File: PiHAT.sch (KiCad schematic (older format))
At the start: 17 parts, among them U1 LM2596T-ADJ

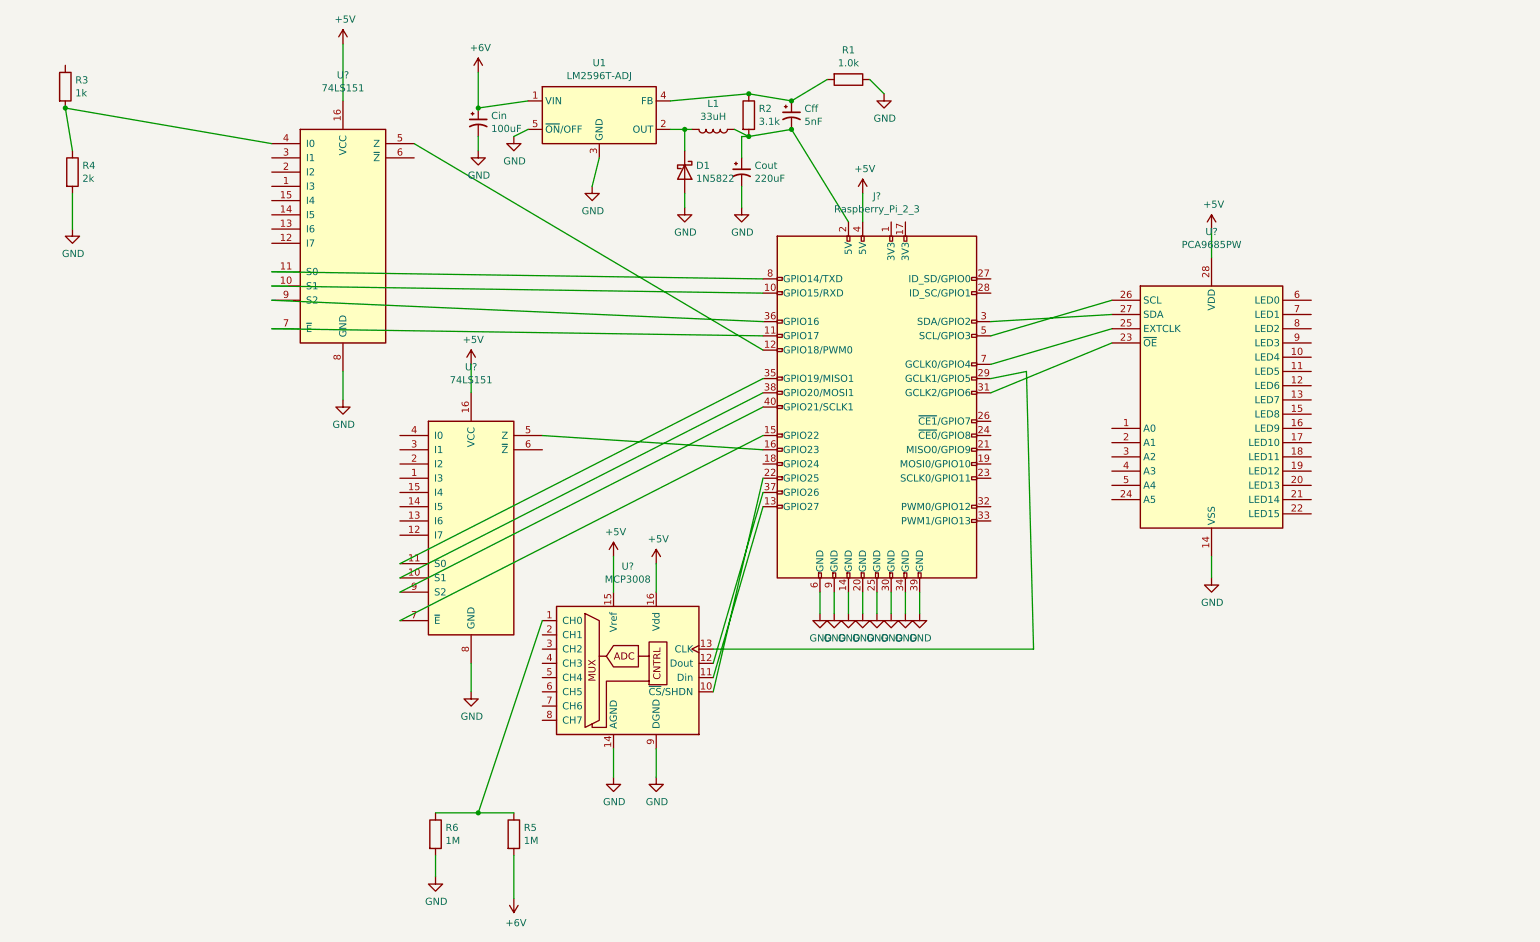
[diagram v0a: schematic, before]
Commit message: Add files via upload
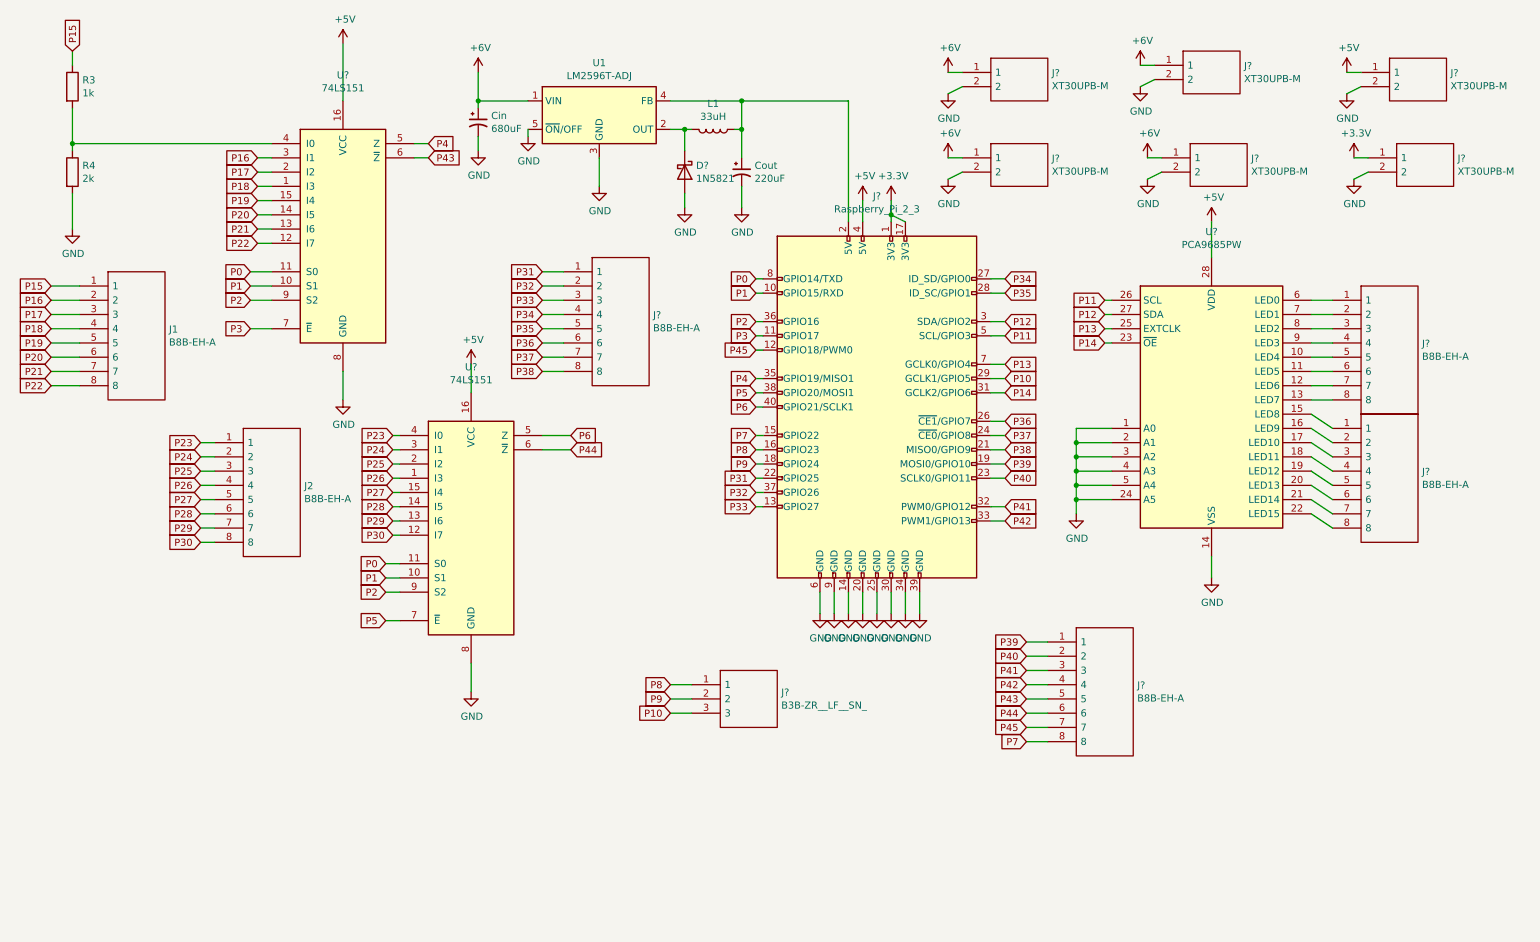
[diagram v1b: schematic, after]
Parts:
- removed Cff: 5nF, symbol Device:CP1_Small
- removed D1: 1N5822, Diode_THT:D_DO-201AD_P15.24mm_Horizontal, symbol Diode:1N5822
- removed R1: 1.0k, symbol Device:R
- removed R2: 3.1k, symbol Device:R
- removed R5, R6: 1M, symbol Device:R
- removed U?: MCP3008, symbol Analog_ADC:MCP3008
- added D?: 1N5821, Diode_THT:D_DO-201AD_P15.24mm_Horizontal, symbol Diode:1N5821
- added J1, J2, J? (x4): B8B-EH-A, SHDR8W64P0X250_1X8_2250X380X600P, symbol SamacSys_Parts:B8B-EH-A
- added J? (x6): XT30UPB-M, SHDR2W160P0X500_1X2_1020X520X1070P, symbol XT30UPB-M:XT30UPB-M
- added J?: B3B-ZR__LF__SN_, SHDR3W50P0X150_1X3_600X350X450P, symbol B3B-ZR__LF__SN_:B3B-ZR__LF__SN_
- Cin: value 100uF -> 680uF
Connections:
- net +5V: now also J?.1
- net +6V: now also J?.1, J?.1, J?.1, J?.1
- net GND: now also U?.1 (A0), U?.2 (A1), U?.24 (A5), U?.3 (A2), U?.4 (A3), U?.5 (A4), D?.2 (A), J?.2, J?.2, J?.2, J?.2, J?.2, J?.2
- net P26: now reaches U?.1 (I3)
- net P26: now also J2.4
- net P1: now reaches U?.10 (S1)
- net P1: now also J?.10 (GPIO15/RXD), U?.10 (S1); no longer J?.38 (GPIO20/MOSI1)
- net P0: now reaches U?.11 (S0)
- net P0: now also J?.8 (GPIO14/TXD), U?.11 (S0); no longer J?.35 (GPIO19/MISO1)
- net P30: now reaches U?.12 (I7)
- net P30: now also J2.8
- net P29: now reaches U?.13 (I6)
- net P29: now also J2.7
- net P28: now reaches U?.14 (I5)
- net P28: now also J2.6
- net P27: now reaches U?.15 (I4)
- net P27: now also J2.5
- net P25: now reaches U?.2 (I2)
- net P25: now also J2.3
- net P24: now reaches U?.3 (I1)
- net P24: now also J2.2
- net P23: now reaches U?.4 (I0)
- net P23: now also J2.1
- net P6: now reaches U?.5 (Z)
- net P6: now also J?.40 (GPIO21/SCLK1); no longer J?.16 (GPIO23)
- net P44: now reaches U?.6 (~Z)
- net P44: now also J?.6
- net P5: now reaches U?.7 (~E)
- net P5: now also J?.38 (GPIO20/MOSI1); no longer J?.15 (GPIO22)
- net P2: now reaches U?.9 (S2)
- net P2: now also J?.36 (GPIO16), U?.9 (S2); no longer J?.40 (GPIO21/SCLK1)
- net P18: now reaches U?.1 (I3)
- net P18: now also J1.4
- net P22: now reaches U?.12 (I7)
- net P22: now also J1.8
- net P21: now reaches U?.13 (I6)
- net P21: now also J1.7
- net P20: now reaches U?.14 (I5)
- net P20: now also J1.6
- net P19: now reaches U?.15 (I4)
- net P19: now also J1.5
- net P17: now reaches U?.2 (I2)
- net P17: now also J1.3
- net P16: now reaches U?.3 (I1)
- net P16: now also J1.2
- net P4: now reaches U?.5 (Z)
- net P4: now also J?.35 (GPIO19/MISO1); no longer J?.12 (GPIO18/PWM0)
- net P43: now reaches U?.6 (~Z)
- net P43: now also J?.5
- net P3: now reaches J?.11 (GPIO17), U?.7 (~E)
- net +3V3: now reaches J?.1 (3V3)
- net +3V3: now also J?.17 (3V3), J?.1
- net P33: now reaches J?.13 (GPIO27)
- net P33: now also J?.3
- net P9: now reaches J?.18 (GPIO24)
- net P9: now also J?.2
- net P39: now reaches J?.19 (MOSI0/GPIO10)
- net P39: now also J?.1
- net at Cout.1, J?.2 (5V), L1.1: now also U1.4 (FB)
- net P38: now reaches J?.21 (MISO0/GPIO9)
- net P38: now also J?.8
- net P31: now reaches J?.22 (GPIO25)
- net P31: now also J?.1
- net P40: now reaches J?.23 (SCLK0/GPIO11)
- net P40: now also J?.2
- net P37: now reaches J?.24 (~CE0~/GPIO8)
- net P37: now also J?.7
- net P36: now reaches J?.26 (~CE1~/GPIO7)
- net P36: now also J?.6
- net P34: now reaches J?.27 (ID_SD/GPIO0)
- net P34: now also J?.4
- net P35: now reaches J?.28 (ID_SC/GPIO1)
- net P35: now also J?.5
- net P10: now reaches J?.29 (GCLK1/GPIO5)
- net P10: now also J?.3
- net P12: now reaches J?.3 (SDA/GPIO2), U?.27 (SDA)
- net P14: now reaches J?.31 (GCLK2/GPIO6), U?.23 (~OE)
- net P41: now reaches J?.32 (PWM0/GPIO12)
- net P41: now also J?.3
- net P42: now reaches J?.33 (PWM1/GPIO13)
- net P42: now also J?.4
- net P32: now reaches J?.37 (GPIO26)
- net P32: now also J?.2
- net P11: now reaches J?.5 (SCL/GPIO3), U?.26 (SCL)
- net P13: now reaches J?.7 (GCLK0/GPIO4), U?.25 (EXTCLK)
- net at L1.2, U1.2 (OUT): now also D?.1 (K)
- net P15: now reaches R3.1
- net P15: now also J1.1
- net at U?.10 (LED4): now also J?.5
- net at U?.11 (LED5): now also J?.6
- net at U?.12 (LED6): now also J?.7
- net at U?.13 (LED7): now also J?.8
- net at U?.15 (LED8): now also J?.1
- net at U?.16 (LED9): now also J?.2
- net at U?.17 (LED10): now also J?.3
- net at U?.18 (LED11): now also J?.4
- net at U?.19 (LED12): now also J?.5
- net at U?.20 (LED13): now also J?.6
- net at U?.21 (LED14): now also J?.7
- net at U?.22 (LED15): now also J?.8
- net at U?.6 (LED0): now also J?.1
- net at U?.7 (LED1): now also J?.2
- net at U?.8 (LED2): now also J?.3
- net at U?.9 (LED3): now also J?.4
- new net P45: J?.12 (GPIO18/PWM0), J?.7
- new net P7: J?.15 (GPIO22), J?.8
- new net P8: J?.1, J?.16 (GPIO23)
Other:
- moved on the sheet: R3
